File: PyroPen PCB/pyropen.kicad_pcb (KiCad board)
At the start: 2 copper layers, 41 x 8 mm, 58 parts, among them J1 AAAA BATT, J2 Front 3.3v LED, J3 MLX90614ESF-DCC-000-TU, J4 BUZZ, J5 DEBUG, SW1 B3U-1000P, U1 ATTINY1616-MNR, U2 MAX17222ELT+T

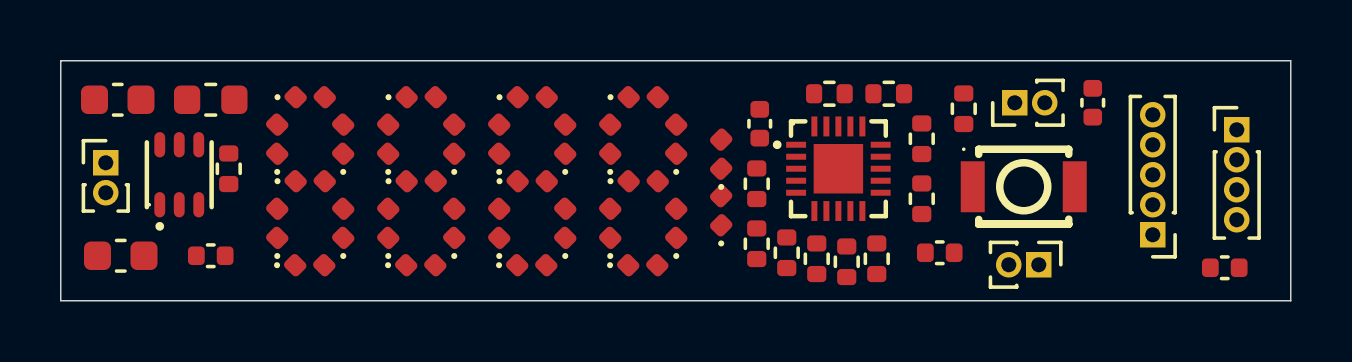
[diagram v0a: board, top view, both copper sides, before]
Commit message: sync
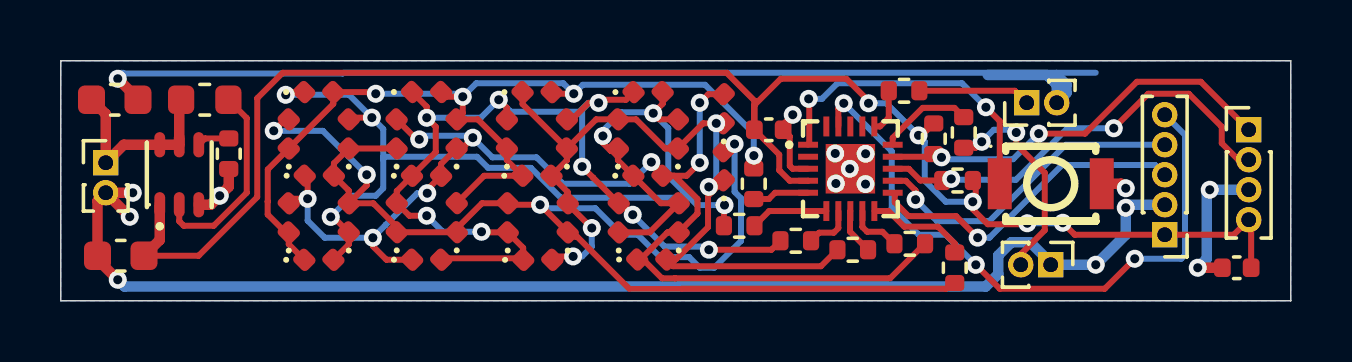
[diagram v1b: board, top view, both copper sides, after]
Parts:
- removed C2, C3, C5: 100nF, Capacitor_SMD:C_0402_1005Metric
- removed R28: 1k, Resistor_SMD:R_0402_1005Metric
- moved D38 3.40 mm to (22.1, 1.60)
- moved R27 2.81 mm to (30.1, 2.39), turned to -90 degrees
- moved R6 2.62 mm to (29.8, 6.90)
- moved R5 2.18 mm to (28.3, 6.10), turned to 180 degrees
- moved R10 2.08 mm to (28.1, 1.00), turned to 180 degrees
- moved R8 1.34 mm to (29.9, 3.99), turned to 180 degrees
- moved R4 1.24 mm to (26.4, 6.30), turned to 0 degrees
- moved SW1 0.91 mm to (33.0, 4.10)
- moved R2 0.84 mm to (22.6, 5.50), turned to 0 degrees
- moved R3 0.50 mm to (24.5, 6.00), turned to 0 degrees
- moved R7 0.50 mm to (5.60, 3.10)
- moved D35 0.42 mm to (7.60, 5.24)
- moved D36 0.42 mm to (7.60, 2.44)
- moved C4 0.40 mm to (39.2, 6.90)
- moved J4 0.40 mm to (33.0, 6.80)
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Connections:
- U1 pad 17: VMON1 -> unconnected-(U1-PC2-Pad17)
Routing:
- net GND: track 0.00 -> 91.1 mm, vias 0 -> 16
- net +3.3V: track 0.00 -> 55.1 mm, vias 0 -> 5
- net Net-(D11-K): track 0.00 -> 43.3 mm, vias 0 -> 4
- net Net-(D10-K): track 0.00 -> 41.5 mm, vias 0 -> 8
- net Net-(D10-A): track 0.00 -> 37.4 mm, vias 0 -> 6
- net Net-(D13-A): track 0.00 -> 32.5 mm, vias 0 -> 8
- net Net-(D2-A): track 0.00 -> 31.5 mm, vias 0 -> 4
- net Net-(D13-K): track 0.00 -> 27.2 mm, vias 0 -> 4
- net UPDI: track 0.00 -> 21.4 mm, vias 0 -> 3
- net SDA: track 0.00 -> 15.0 mm, vias 0 -> 2
- net SCL: track 0.00 -> 13.7 mm, vias 0 -> 2
- net RX: track 0.00 -> 11.0 mm, vias 0 -> 1
- net TX: track 0.00 -> 10.9 mm, vias 0 -> 1
- net WAKE_BTN: track 0.00 -> 10.8 mm, vias 0 -> 2
- net Net-(J4-Pin_2): track 0.00 -> 7.17 mm, vias 0 -> 2
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- added copper zone on B.Cu, net GND

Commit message: sync
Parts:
- R7: value 80k -> 80.6k
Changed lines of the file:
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@@
 			(net "unconnected-(U1-EXTCLK{slash}PA3-Pad2)")
 			(pinfunction "EXTCLK/PA3_2")
-			(pintype "unspecified+no_connect")
+			(pintype "unspecified")
 		)
 		(pad "3" smd rect
@@
 			(net "unconnected-(U1-PC2-Pad17)")
 			(pinfunction "PC2_17")
-			(pintype "unspecified+no_connect")
+			(pintype "unspecified")
 		)
 		(pad "18" smd rect
@@
 			(net "unconnected-(U1-PC3-Pad18)")
 			(pinfunction "PC3_18")
-			(pintype "unspecified+no_connect")
+			(pintype "unspecified")
 		)
 		(pad "19" smd rect
@@
 			(net "unconnected-(U1-PA1-Pad20)")
 			(pinfunction "PA1_20")
-			(pintype "unspecified+no_connect")
+			(pintype "unspecified")
 		)
 		(pad "21" smd rect
@@
 			)
 		)
-		(property "Value" "80k"
+		(property "Value" "80.6k"
 			(at -0.000001 1.169999 90)
 			(layer "F.Fab")
@@
 	)
 	(segment
+		(start 27.73125 2.56875)
+		(end 28.73 1.57)
+		(width 0.2)
+		(layer "F.Cu")
+		(net "BUZZ")
+	)
+	(segment
+		(start 28.73 1.57)
+		(end 29.789998 1.57)
+		(width 0.2)
+		(layer "F.Cu")
+		(net "BUZZ")
+	)
+	(segment
+		(start 29.789998 1.57)
+		(end 30.1 1.880002)
+		(width 0.2)
+		(layer "F.Cu")
+		(net "BUZZ")
+	)
+	(segment
+		(start 27.73125 2.800005)
+		(end 27.73125 2.56875)
+		(width 0.2)
+		(layer "F.Cu")
+		(net "BUZZ")
+	)
+	(segment
+		(start 31.85 2.392558)
+		(end 31.85 2.787337)
+		(width 0.2)
+		(layer "F.Cu")
+		(net "Net-(J4-Pin_2)")
+	)
+	(segment
+		(start 31.85 2.787337)
+		(end 32.8 3.737337)
+		(width 0.2)
+		(layer "F.Cu")
+		(net "Net-(J4-Pin_2)")
+	)
+	(segment
+		(start 32.8 3.737337)
+		(end 32.8 5.649998)
+		(width 0.2)
+		(layer "F.Cu")
+		(net "Net-(J4-Pin_2)")
+	)
+	(segment
+		(start 32 6.449998)
+		(end 32 6.8)
+		(width 0.2)
+		(layer "F.Cu")
+		(net "Net-(J4-Pin_2)")
+	)
+	(segment
+		(start 32.8 5.649998)
+		(end 32 6.449998)
+		(width 0.2)
+		(layer "F.Cu")
+		(net "Net-(J4-Pin_2)")
+	)
+	(segment
+		(start 30.5 2.9)
+		(end 30.7 2.7)
+		(width 0.2)
+		(layer "F.Cu")
+		(net "Net-(J4-Pin_2)")
+	)
+	(segment
+		(start 30.1 2.9)
+		(end 30.5 2.9)
+		(width 0.2)
+		(layer "F.Cu")
+		(net "Net-(J4-Pin_2)")
+	)
+	(via
+		(at 30.7 2.7)
+		(size 0.6)
+		(drill 0.3)
+		(layers "F.Cu" "B.Cu")
+		(net "Net-(J4-Pin_2)")
+	)
+	(via
+		(at 31.85 2.392558)
+		(size 0.6)
+		(drill 0.3)
+		(layers "F.Cu" "B.Cu")
+		(net "Net-(J4-Pin_2)")
+	)
+	(segment
+		(start 31.757442 2.3)
+		(end 31.1 2.3)
+		(width 0.2)
+		(layer "B.Cu")
+		(net "Net-(J4-Pin_2)")
+	)
+	(segment
+		(start 31.85 2.392558)
+		(end 31.757442 2.3)
+		(width 0.2)
+		(layer "B.Cu")
+		(net "Net-(J4-Pin_2)")
+	)
+	(segment
+		(start 31.1 2.3)
+		(end 30.7 2.7)
+		(width 0.2)
+		(layer "B.Cu")
+		(net "Net-(J4-Pin_2)")
+	)
+	(segment
+		(start 2.1 2.8)
+		(end 1.5 3.4)
+		(width 0.35)
+		(layer "F.Cu")
+		(net "+VBAT")
+	)
+	(segment
+		(start 3.95 1.3625)
+		(end 4.0125 1.3)
+		(width 0.35)
+		(layer "F.Cu")
+		(net "+VBAT")
+	)
+	(segment
+		(start 3.3 2.8)
+		(end 3.95 2.8)
+		(width 0.35)
+		(layer "F.Cu")
+		(net "+VBAT")
+	)
+	(segment
+		(start 1.5 3.4)
+		(end 1.5 1.775006)
+		(width 0.35)
+		(layer "F.Cu")
+		(net "+VBAT")
+	)
+	(segment
+		(start 3.95 2.8)
+		(end 3.95 1.3625)
+		(width 0.35)
+		(layer "F.Cu")
+		(net "+VBAT")
+	)
+	(segment
+		(start 3.3 2.8)
+		(end 2.1 2.8)
+		(width 0.35)
+		(layer "F.Cu")
+		(net "+VBAT")
+	)
+	(segment
+		(start 1.5 1.775006)
+		(end 1.024999 1.300005)
+		(width 0.35)
+		(layer "F.Cu")
+		(net "+VBAT")
+	)
+	(segment
+		(start 4.1 5.5)
+		(end 5.1 5.5)
+		(width 0.2)
+		(layer "F.Cu")
+		(net "Net-(U2-LX)")
+	)
+	(segment
+		(start 3.95 4.8)
+		(end 3.95 5.35)
+		(width 0.2)
+		(layer "F.Cu")
+		(net "Net-(U2-LX)")
+	)
+	(segment
+		(start 5.1 5.5)
+		(end 6.2 4.4)
+		(width 0.2)
+		(layer "F.Cu")
+		(net "Net-(U2-LX)")
+	)
+	(segment
+		(start 6.2 4.4)
+		(end 6.2 1.9125)
+		(width 0.2)
+		(layer "F.Cu")
+		(net "Net-(U2-LX)")
+	)
+	(segment
+		(start 6.2 1.9125)
+		(end 5.5875 1.3)
+		(width 0.2)
+		(layer "F.Cu")
+		(net "Net-(U2-LX)")
+	)
+	(segment
+		(start 3.95 5.35)
+		(end 4.1 5.5)
+		(width 0.2)
+		(layer "F.Cu")
+		(net "Net-(U2-LX)")
+	)
+	(segment
 		(start 30.4 4.7)
 		(end 30.5 4.6)
@@
 	)
 	(segment
-		(start 27.73125 2.56875)
-		(end 28.73 1.57)
-		(width 0.2)
-		(layer "F.Cu")
-		(net "BUZZ")
-	)
-	(segment
-		(start 28.73 1.57)
-		(end 29.789998 1.57)
-		(width 0.2)
-		(layer "F.Cu")
-		(net "BUZZ")
-	)
-	(segment
-		(start 29.789998 1.57)
-		(end 30.1 1.880002)
-		(width 0.2)
-		(layer "F.Cu")
-		(net "BUZZ")
-	)
-	(segment
-		(start 27.73125 2.800005)
-		(end 27.73125 2.56875)
-		(width 0.2)
-		(layer "F.Cu")
-		(net "BUZZ")
-	)
-	(segment
-		(start 31.85 2.392558)
-		(end 31.85 2.787337)
-		(width 0.2)
-		(layer "F.Cu")
-		(net "Net-(J4-Pin_2)")
-	)
-	(segment
-		(start 31.85 2.787337)
-		(end 32.8 3.737337)
-		(width 0.2)
-		(layer "F.Cu")
-		(net "Net-(J4-Pin_2)")
-	)
-	(segment
-		(start 32.8 3.737337)
-		(end 32.8 5.649998)
-		(width 0.2)
-		(layer "F.Cu")
-		(net "Net-(J4-Pin_2)")
-	)
-	(segment
-		(start 32 6.449998)
-		(end 32 6.8)
-		(width 0.2)
-		(layer "F.Cu")
-		(net "Net-(J4-Pin_2)")
-	)
-	(segment
-		(start 32.8 5.649998)
-		(end 32 6.449998)
-		(width 0.2)
-		(layer "F.Cu")
-		(net "Net-(J4-Pin_2)")
-	)
-	(segment
-		(start 30.5 2.9)
-		(end 30.7 2.7)
-		(width 0.2)
-		(layer "F.Cu")
-		(net "Net-(J4-Pin_2)")
-	)
-	(segment
-		(start 30.1 2.9)
-		(end 30.5 2.9)
-		(width 0.2)
-		(layer "F.Cu")
-		(net "Net-(J4-Pin_2)")
-	)
-	(via
-		(at 30.7 2.7)
-		(size 0.6)
-		(drill 0.3)
-		(layers "F.Cu" "B.Cu")
-		(net "Net-(J4-Pin_2)")
-	)
-	(via
-		(at 31.85 2.392558)
-		(size 0.6)
-		(drill 0.3)
-		(layers "F.Cu" "B.Cu")
-		(net "Net-(J4-Pin_2)")
-	)
-	(segment
-		(start 31.757442 2.3)
-		(end 31.1 2.3)
-		(width 0.2)
-		(layer "B.Cu")
-		(net "Net-(J4-Pin_2)")
-	)
-	(segment
-		(start 31.85 2.392558)
-		(end 31.757442 2.3)
-		(width 0.2)
-		(layer "B.Cu")
-		(net "Net-(J4-Pin_2)")
-	)
-	(segment
-		(start 31.1 2.3)
-		(end 30.7 2.7)
-		(width 0.2)
-		(layer "B.Cu")
-		(net "Net-(J4-Pin_2)")
-	)
-	(segment
-		(start 2.1 2.8)
-		(end 1.5 3.4)
-		(width 0.35)
-		(layer "F.Cu")
-		(net "+VBAT")
-	)
-	(segment
-		(start 3.95 1.3625)
-		(end 4.0125 1.3)
-		(width 0.35)
-		(layer "F.Cu")
-		(net "+VBAT")
-	)
-	(segment
-		(start 3.3 2.8)
-		(end 3.95 2.8)
-		(width 0.35)
-		(layer "F.Cu")
-		(net "+VBAT")
-	)
-	(segment
-		(start 1.5 3.4)
-		(end 1.5 1.775006)
-		(width 0.35)
-		(layer "F.Cu")
-		(net "+VBAT")
-	)
-	(segment
-		(start 3.95 2.8)
-		(end 3.95 1.3625)
-		(width 0.35)
-		(layer "F.Cu")
-		(net "+VBAT")
-	)
-	(segment
-		(start 3.3 2.8)
-		(end 2.1 2.8)
-		(width 0.35)
-		(layer "F.Cu")
-		(net "+VBAT")
-	)
-	(segment
-		(start 1.5 1.775006)
-		(end 1.024999 1.300005)
-		(width 0.35)
-		(layer "F.Cu")
-		(net "+VBAT")
-	)
-	(segment
-		(start 4.1 5.5)
-		(end 5.1 5.5)
-		(width 0.2)
-		(layer "F.Cu")
-		(net "Net-(U2-LX)")
-	)
-	(segment
-		(start 3.95 4.8)
-		(end 3.95 5.35)
-		(width 0.2)
-		(layer "F.Cu")
-		(net "Net-(U2-LX)")
-	)
-	(segment
-		(start 5.1 5.5)
-		(end 6.2 4.4)
-		(width 0.2)
-		(layer "F.Cu")
-		(net "Net-(U2-LX)")
-	)
-	(segment
-		(start 6.2 4.4)
-		(end 6.2 1.9125)
-		(width 0.2)
-		(layer "F.Cu")
-		(net "Net-(U2-LX)")
-	)
-	(segment
-		(start 6.2 1.9125)
-		(end 5.5875 1.3)
-		(width 0.2)
-		(layer "F.Cu")
-		(net "Net-(U2-LX)")
-	)
-	(segment
-		(start 3.95 5.35)
-		(end 4.1 5.5)
-		(width 0.2)
-		(layer "F.Cu")
-		(net "Net-(U2-LX)")
-	)
-	(segment
